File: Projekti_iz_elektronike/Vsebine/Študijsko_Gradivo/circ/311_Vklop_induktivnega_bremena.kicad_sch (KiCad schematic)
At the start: 8 parts, among them Q1 BC108

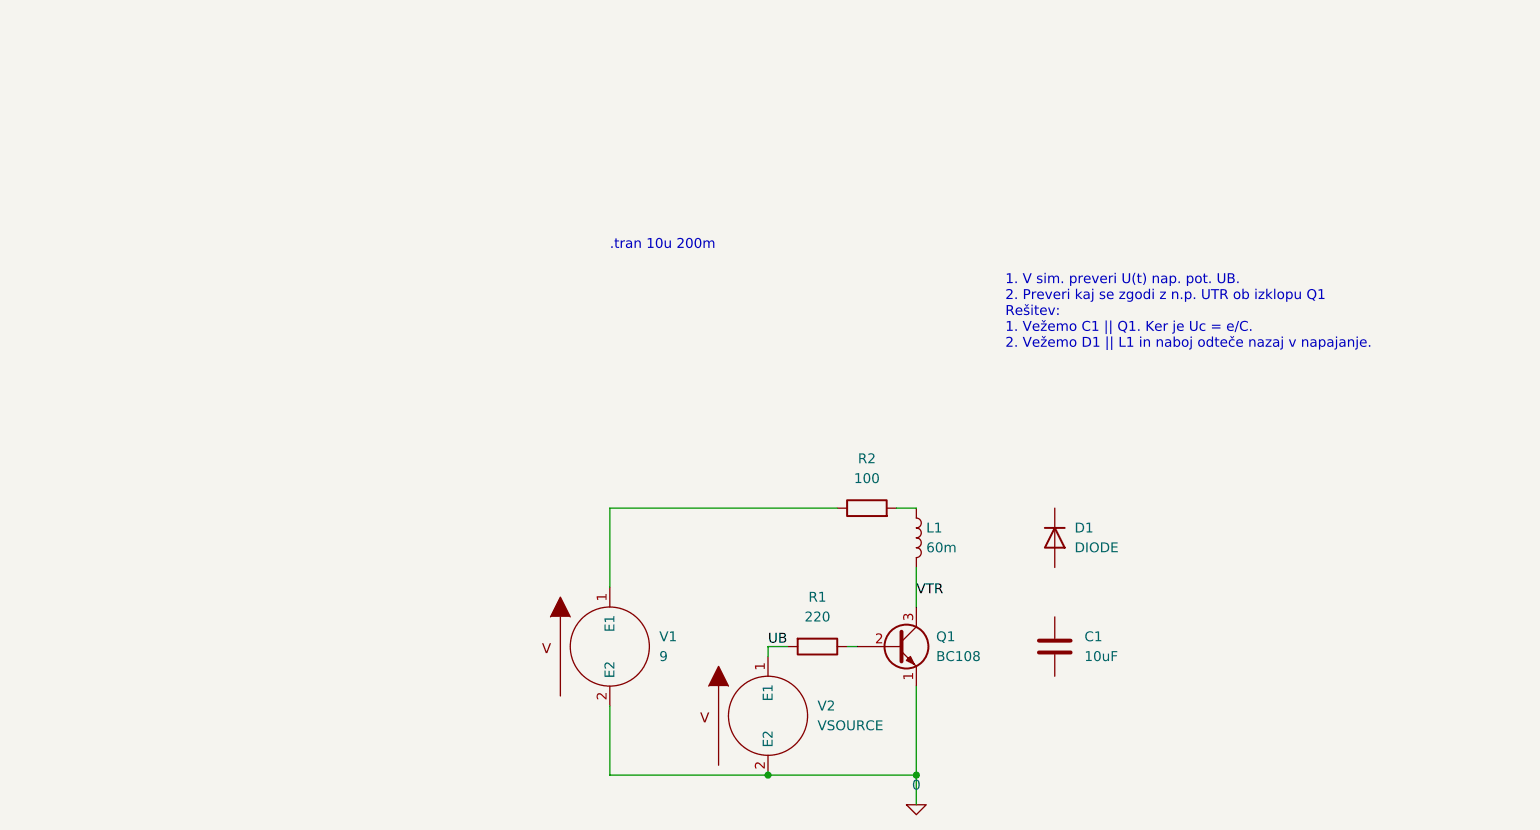
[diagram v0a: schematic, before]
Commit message: popravljena vezja
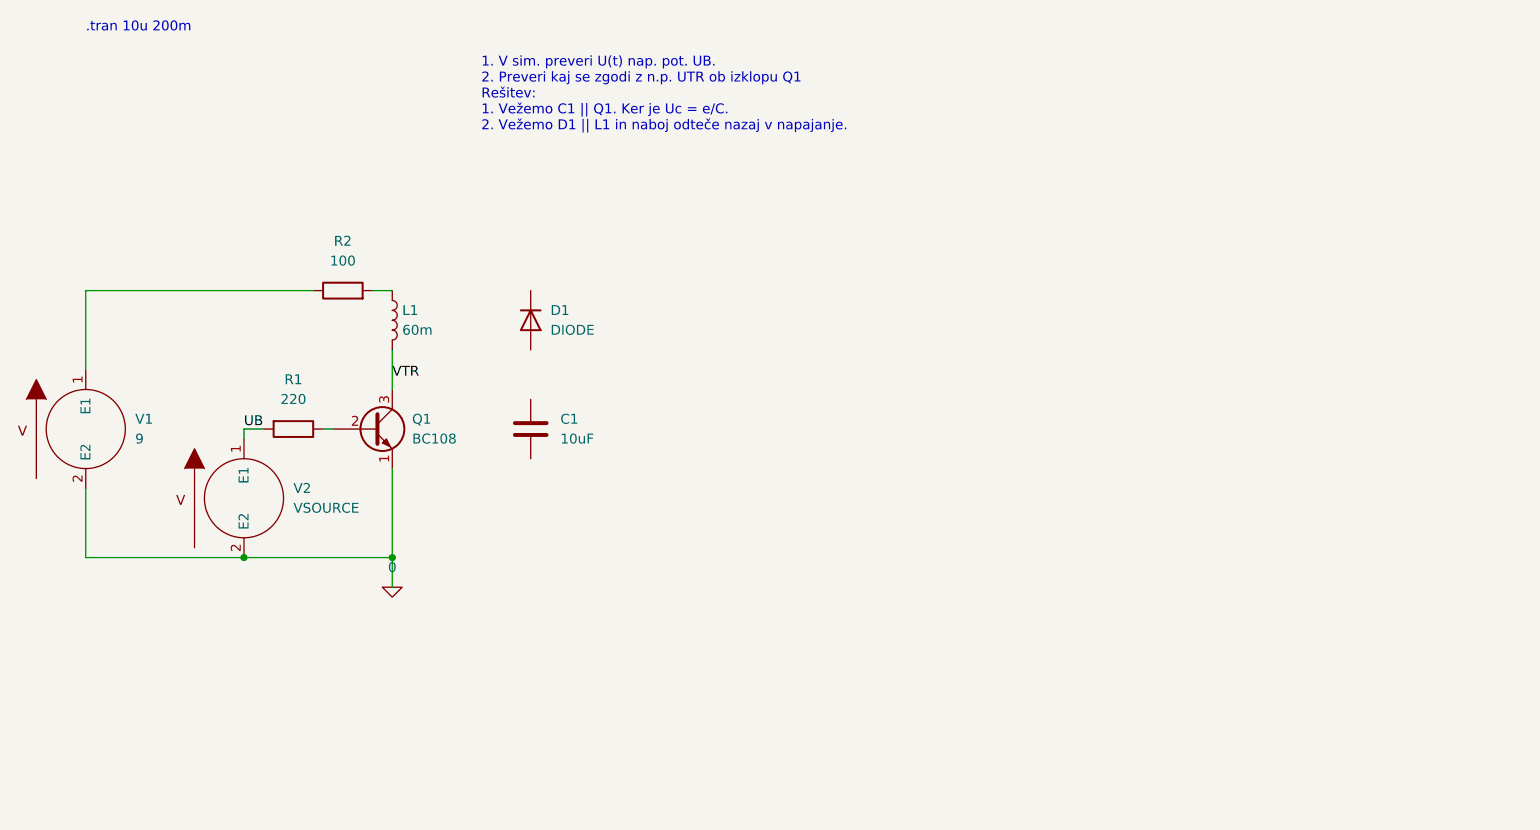
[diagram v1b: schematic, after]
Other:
- moved on the sheet: C1, D1, L1, Q1, R1, R2, V1, V2
